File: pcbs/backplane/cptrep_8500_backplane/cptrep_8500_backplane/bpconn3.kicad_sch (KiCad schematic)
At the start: 1 part, among them J3 cpt-backplane_100

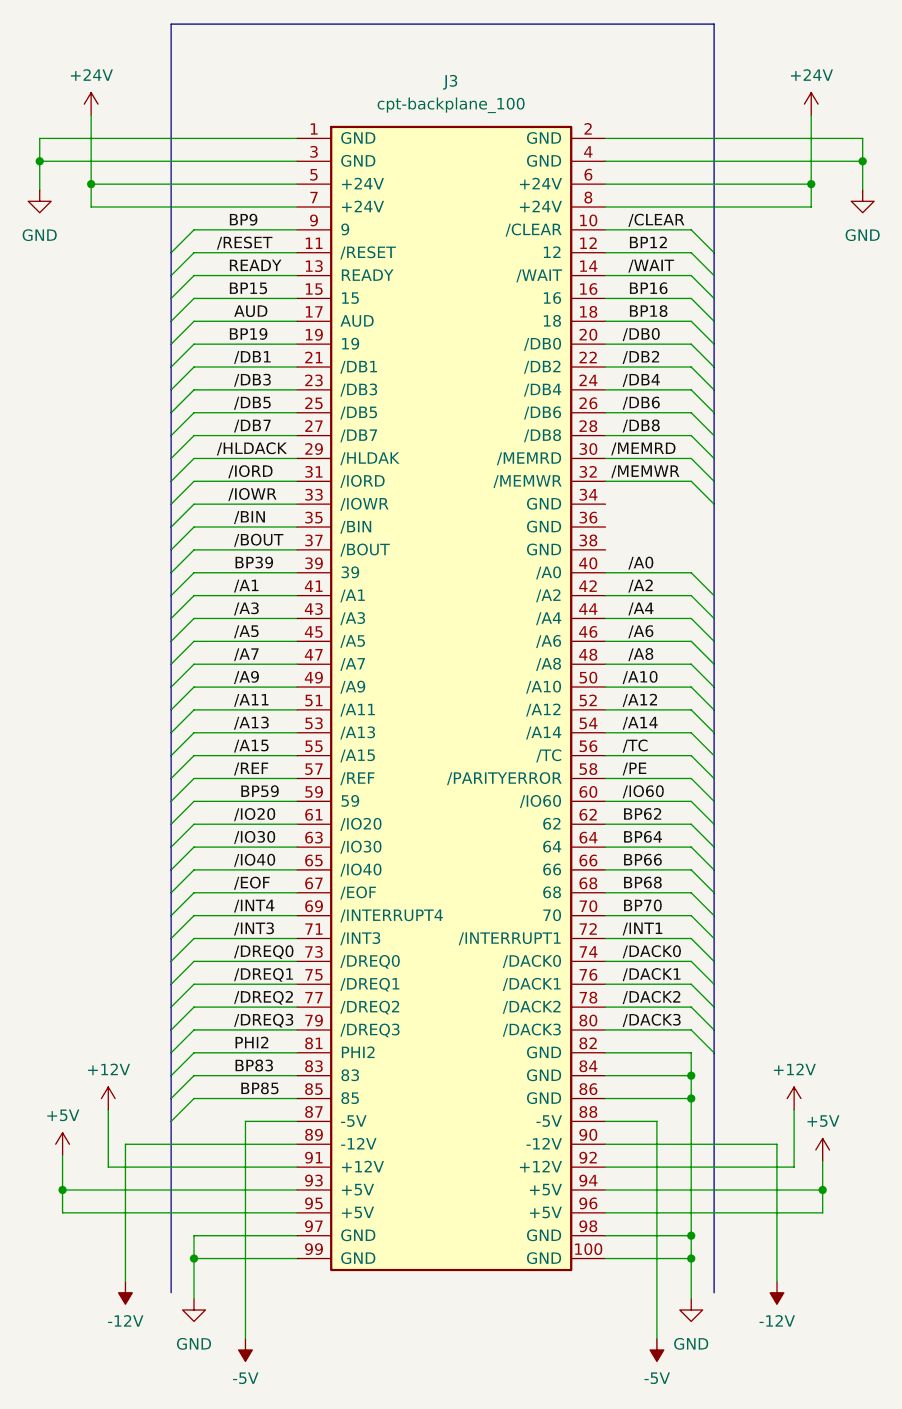
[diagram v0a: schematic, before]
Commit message: "Update"
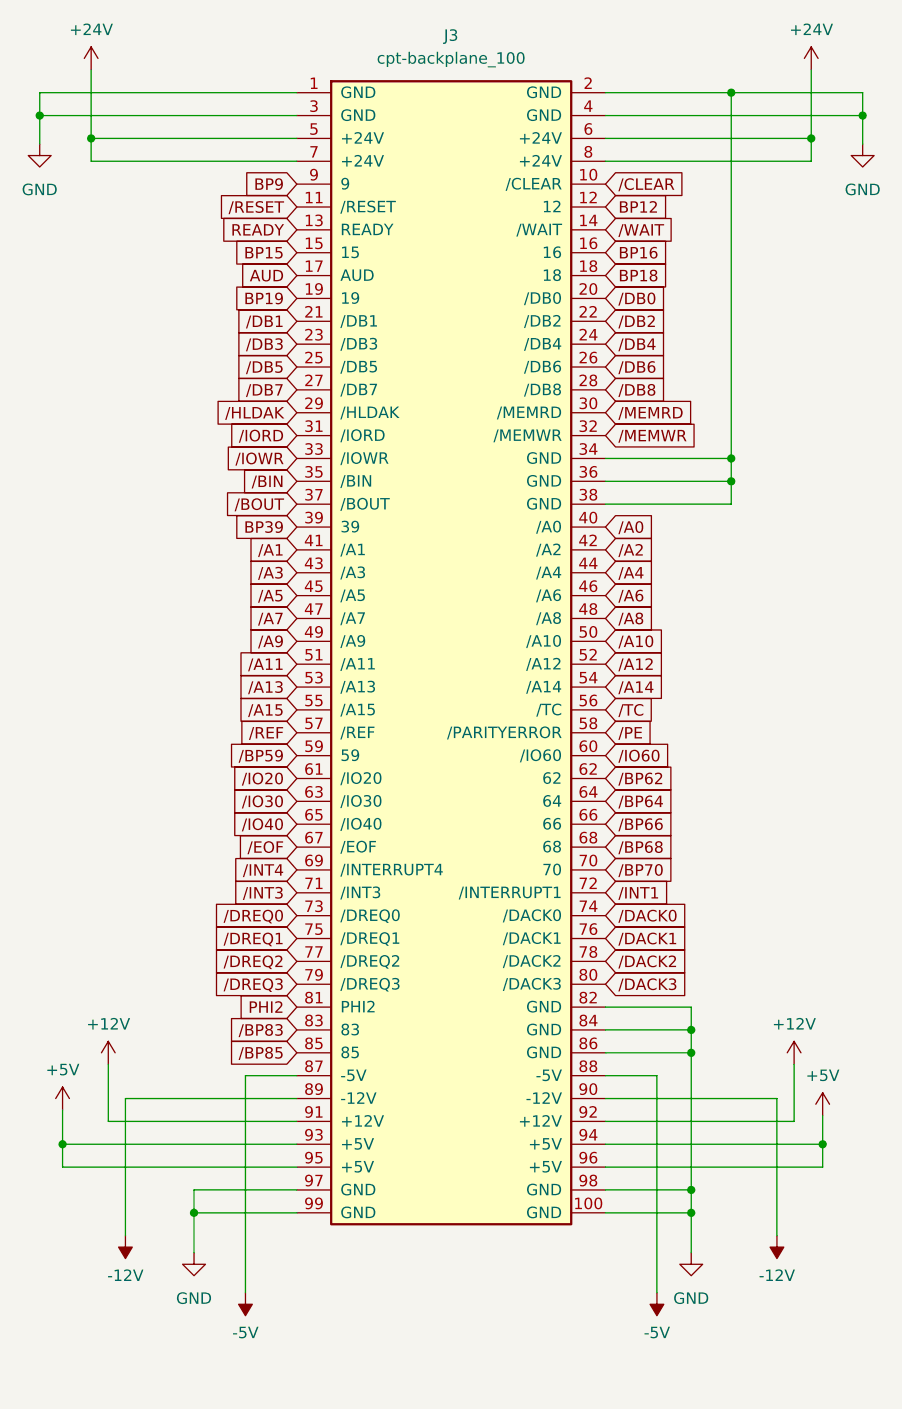
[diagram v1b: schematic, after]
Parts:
- J3: footprint (none) -> ajm-cpt:cpt-8500-backplane-connector
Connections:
- net GND: now also J3.34 (GND), J3.36 (GND), J3.38 (GND)
- net /BP68: now reaches J3.68
- net BP59 renamed /BP59
- net BP62 renamed /BP62
- net BP64 renamed /BP64
- net BP66 renamed /BP66
- net BP70 renamed /BP70
- net BP83 renamed /BP83
- net BP85 renamed /BP85
- net /HLDACK renamed /HLDAK
